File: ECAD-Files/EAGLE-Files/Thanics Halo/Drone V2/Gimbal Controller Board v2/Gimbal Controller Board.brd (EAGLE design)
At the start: 38.8 x 28.2 mm, 66 parts, among them J3 GIMBAL_POWER_CONNECTOR, J4 SERVO_CONNECTOR, J5 SERVO_CONNECTOR, J8 USB_MICRO_B_SMT, U1 TPS65261RHBR, U2 DRV8839DSSR, U4 CP2102-GMRQFN28_5X5-M, U5 DRV8839DSSR, U6 DRV8839DSSR, U7 STM32F303, U8 ATSHA204A, U9 CAT24C256

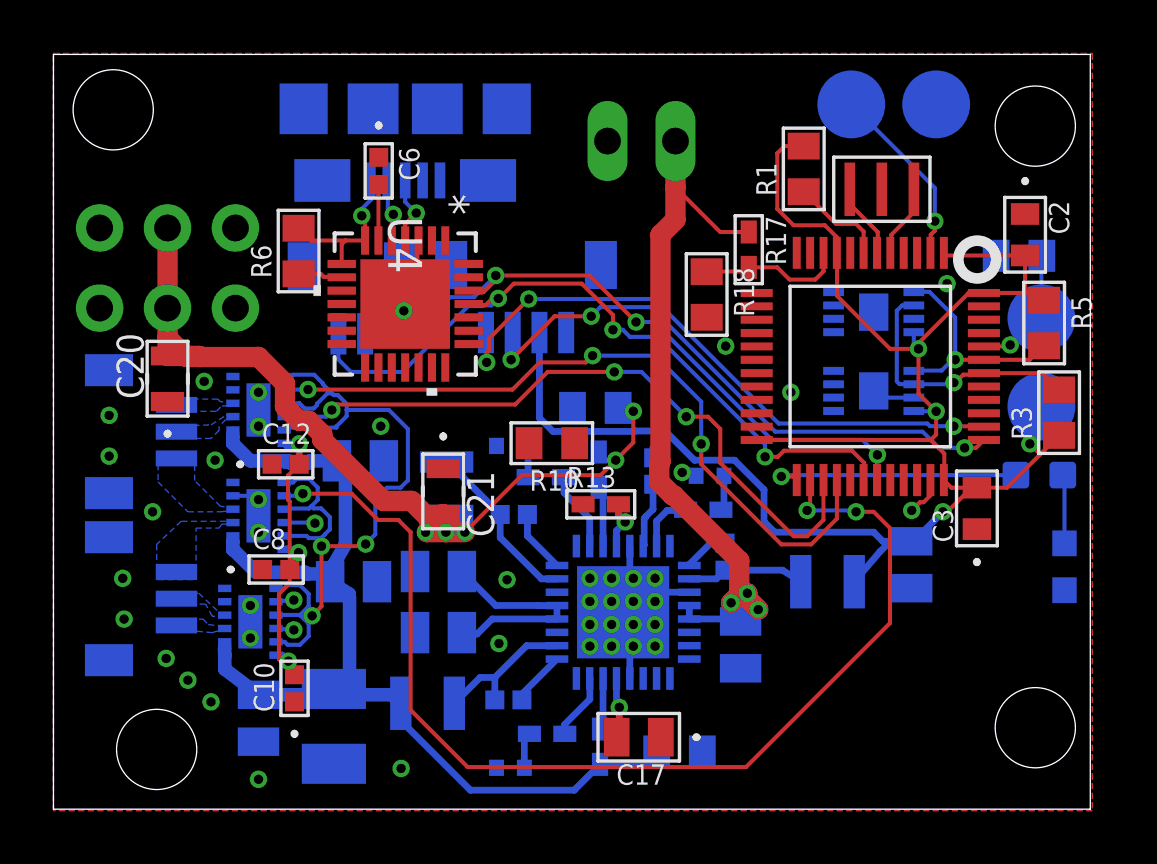
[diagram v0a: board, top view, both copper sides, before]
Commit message: Started V3 Design
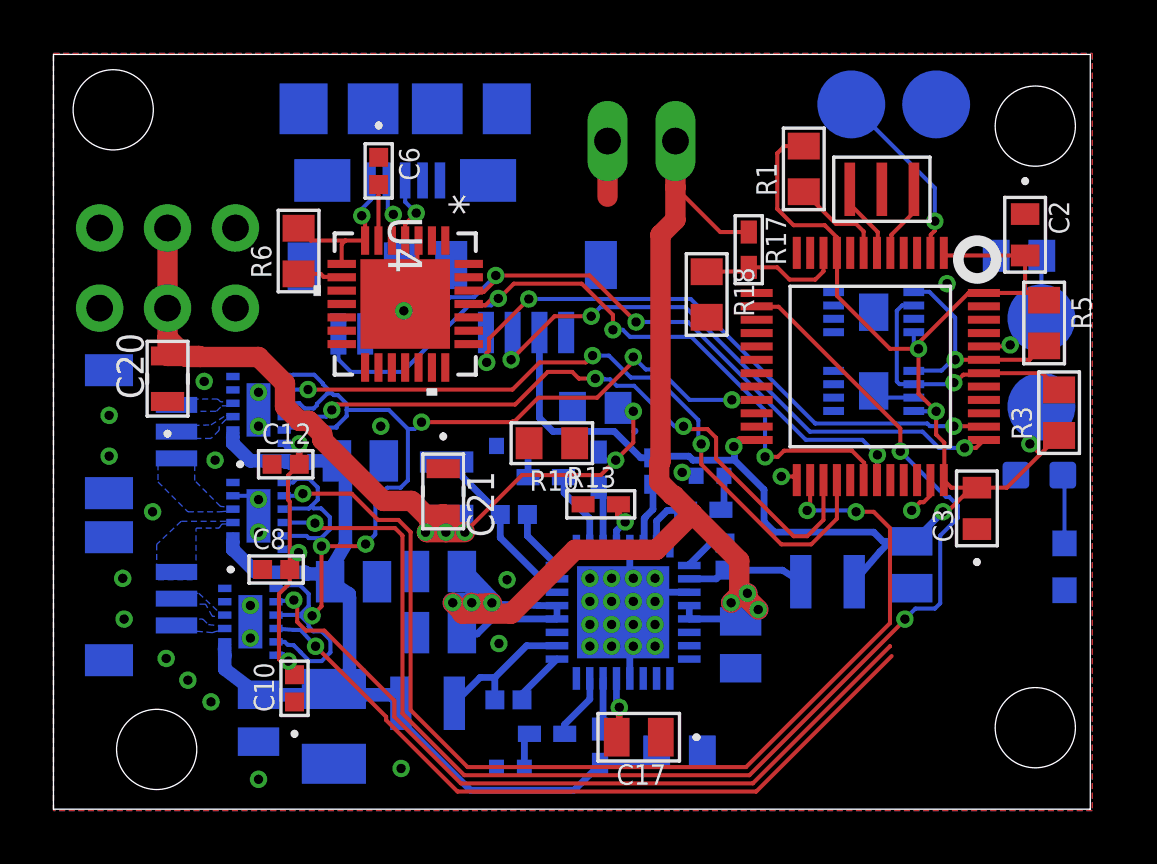
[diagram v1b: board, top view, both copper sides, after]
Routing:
- net TIM3_CH2: track 1.17 -> 50.1 mm, vias 1 -> 3
- net TIM3_CH4: track 0.67 -> 28.7 mm
- net TIM3_CH3: track 0.67 -> 27.7 mm
- net EN_MOTOR: track 33.1 -> 50.2 mm, vias 3 -> 6
- net V_BATT: track 35.6 -> 49.0 mm, vias 3 -> 6
- net LED: track 9.43 -> 0.71 mm
- net +3V3: track 82.3 -> 76.4 mm, vias 7 -> 8
- net GND: track 10.7 -> 12.7 mm, vias 43 -> 41
- net USART1_TX: track 27.6 -> 28.4 mm
